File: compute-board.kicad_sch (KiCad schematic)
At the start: 5 parts, among them J1 PC104

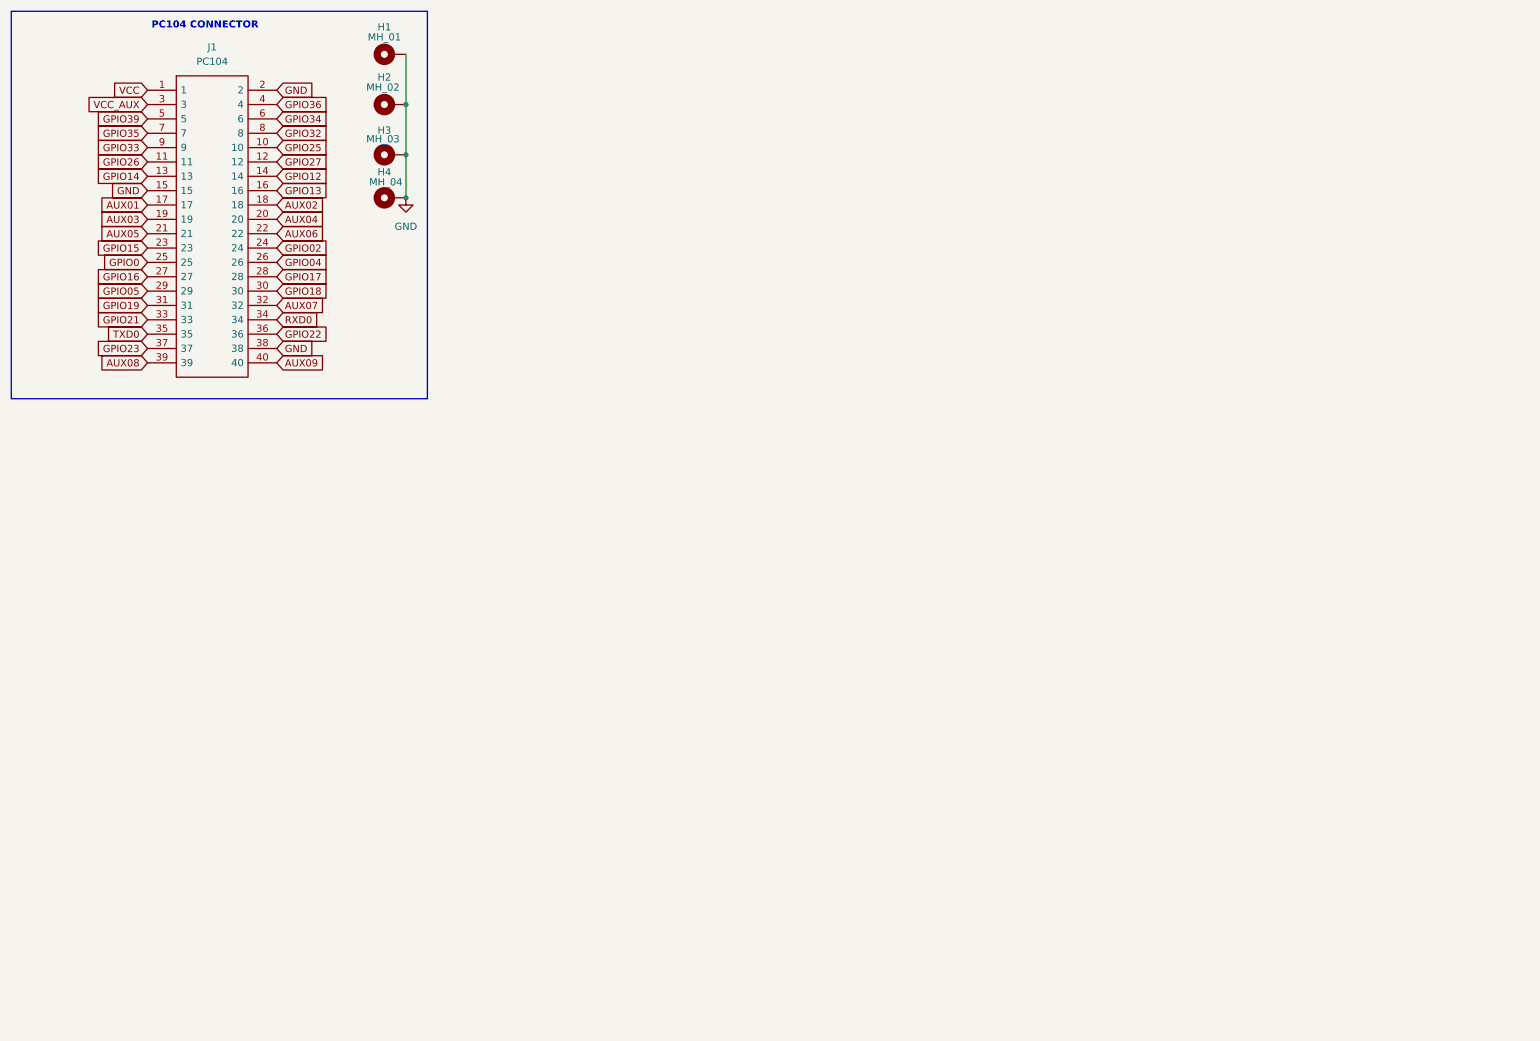
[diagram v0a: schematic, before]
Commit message: Initial commit
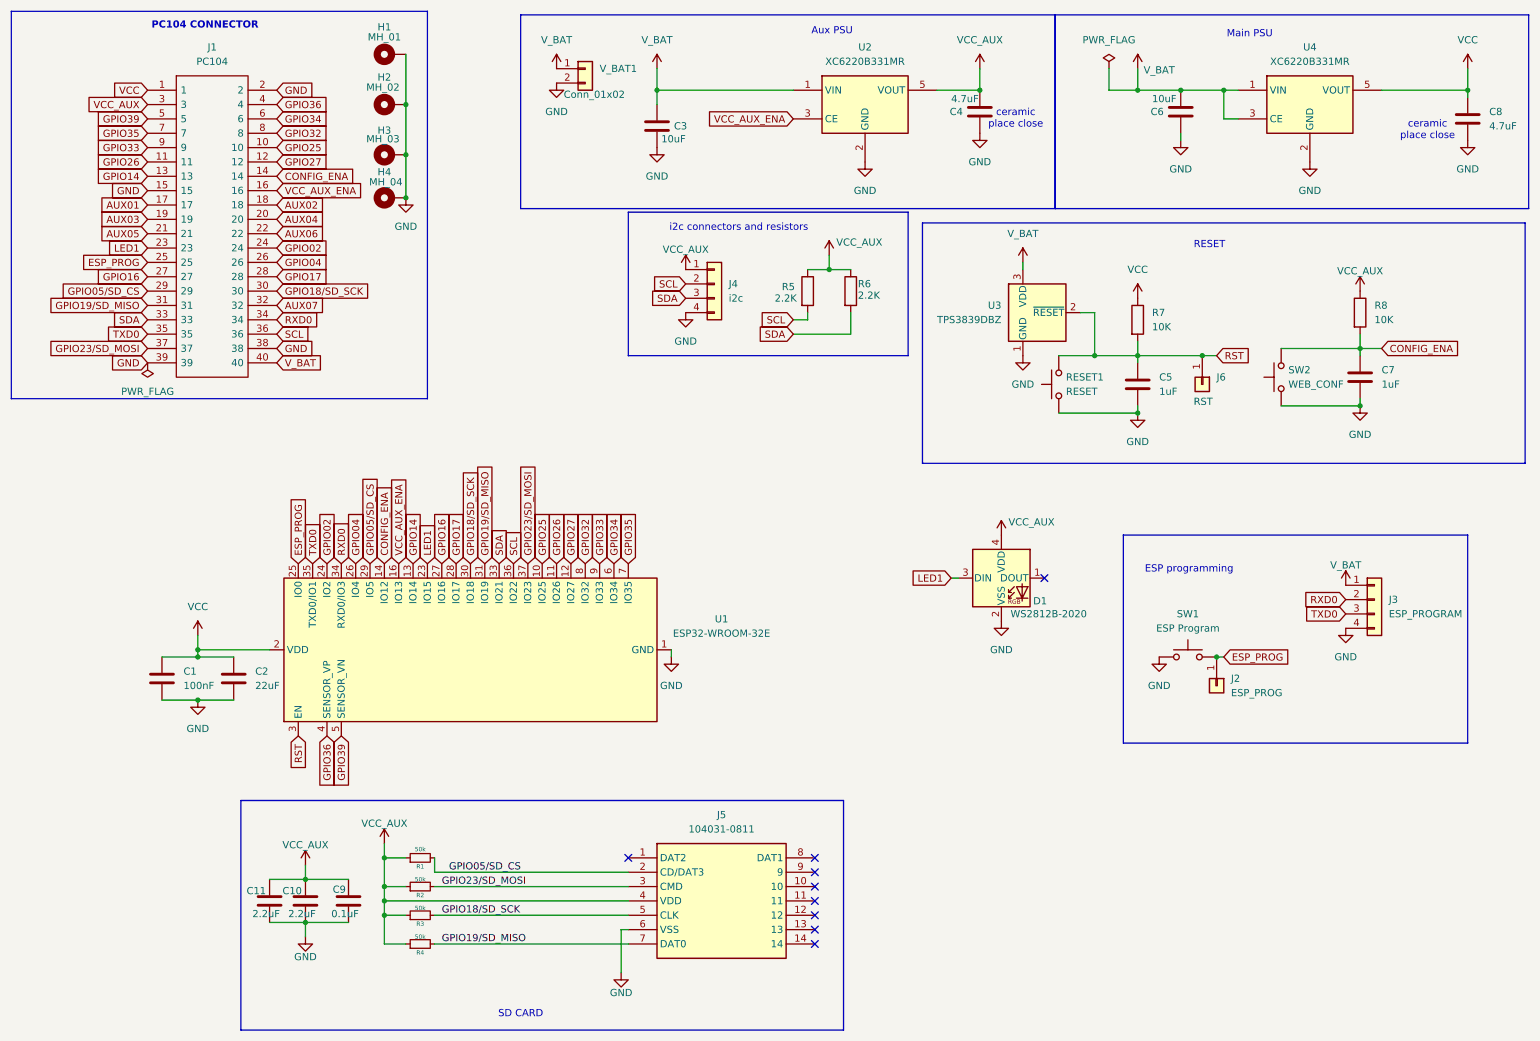
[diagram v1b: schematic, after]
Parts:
- added C1: 100nF, Capacitor_SMD:C_1206_3216Metric_Pad1.33x1.80mm_HandSolder, symbol Device:C
- added C10, C11: 2.2uF, Capacitor_SMD:C_1206_3216Metric_Pad1.33x1.80mm_HandSolder, symbol Device:C
- added C2: 22uF, Capacitor_Tantalum_SMD:CP_EIA-3528-21_Kemet-B_HandSolder, symbol Device:C
- added C3, C6: 10uF, Capacitor_SMD:C_1206_3216Metric_Pad1.33x1.80mm_HandSolder, symbol Device:C
- added C4, C8: 4.7uF, Capacitor_SMD:C_1206_3216Metric_Pad1.33x1.80mm_HandSolder, symbol Device:C
- added C5, C7: 1uF, Capacitor_SMD:C_1206_3216Metric_Pad1.33x1.80mm_HandSolder, symbol Device:C
- added C9: 0.1uF, Capacitor_SMD:C_1206_3216Metric_Pad1.33x1.80mm_HandSolder, symbol Device:C
- added D1: WS2812B-2020, LED_SMD:LED_WS2812B-2020_PLCC4_2.0x2.0mm, symbol LED:WS2812B-2020
- added J2: ESP_PROG, TestPoint:TestPoint_Pad_2.0x2.0mm, symbol Connector_Generic:Conn_01x01
- added J3: ESP_PROGRAM, Connector_JST:JST_XH_B4B-XH-AM_1x04_P2.50mm_Vertical, symbol Connector_Generic:Conn_01x04
- added J4: i2c, Connector_JST:JST_XH_B4B-XH-AM_1x04_P2.50mm_Vertical, symbol Connector_Generic:Conn_01x04
- added J5: 104031-0811, Project-Specific:1040310811, symbol MOLEX 1040310811:104031-0811
- added J6: RST, TestPoint:TestPoint_Pad_2.0x2.0mm, symbol Connector_Generic:Conn_01x01
- added R1, R2, R3, R4: 50k, Resistor_SMD:R_1206_3216Metric_Pad1.30x1.75mm_HandSolder, symbol Device:R_Small
- added R5, R6: 2.2K, Resistor_SMD:R_1206_3216Metric_Pad1.30x1.75mm_HandSolder, symbol Device:R
- added R7, R8: 10K, Resistor_SMD:R_1206_3216Metric_Pad1.30x1.75mm_HandSolder, symbol Device:R
- added RESET1: RESET, Button_Switch_SMD:SW_Push_1P1T_XKB_TS-1187A, symbol Switch:SW_Push
- added SW1: ESP Program, Button_Switch_SMD:SW_Push_1P1T_XKB_TS-1187A, symbol Switch:SW_Push
- added SW2: WEB_CONF, Button_Switch_SMD:SW_Push_1P1T_XKB_TS-1187A, symbol Switch:SW_Push
- added U1: ESP32-WROOM-32E, RF_Module:ESP32-WROOM-32D, symbol RF_Module:ESP32-WROOM-32E
- added U2, U4: XC6220B331MR, Package_TO_SOT_SMD:SOT-23-5, symbol Regulator_Linear:XC6220B331MR
- added U3: TPS3839DBZ, Package_TO_SOT_SMD:SOT-23, symbol Power_Supervisor:TPS3839DBZ
- added V_BAT1: Conn_01x02, TerminalBlock_Altech:Altech_AK300_1x02_P5.00mm_45-Degree, symbol Connector_Generic:Conn_01x02
- J1: footprint RHDR40W66P254_2X20_5146X500X1105P -> Project-Specific:RHDR40W66P254_2X20_5146X500X1105P
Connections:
- net AUX08 is gone; now on net GND: J1.39
- net GND: now also C1.2, C10.2, C11.2, C2.2, C3.1, C4.2, C5.2, C6.2, C7.2, C8.2, C9.2, D1.2 (VSS), J3.4 (Pin_4), J4.4 (Pin_4), J5.6 (VSS), RESET1.1, SW1.1, SW2.1, U1.1 (GND), U1.15 (GND), U1.38 (GND), U1.39 (GND), U2.2 (GND), U3.1 (GND), U4.2 (GND), V_BAT1.2 (Pin_2)
- net GPIO02: now also U1.24 (IO2)
- net GPIO04: now also U1.26 (IO4)
- net GPIO14: now also U1.13 (IO14)
- net GPIO16: now also U1.27 (IO16)
- net GPIO17: now also U1.28 (IO17)
- net GPIO25: now also U1.10 (IO25)
- net GPIO26: now also U1.11 (IO26)
- net GPIO27: now also U1.12 (IO27)
- net GPIO32: now also U1.8 (IO32)
- net GPIO33: now also U1.9 (IO33)
- net GPIO34: now also U1.6 (IO34)
- net GPIO35: now also U1.7 (IO35)
- net GPIO36: now also U1.4 (SENSOR_VP)
- net GPIO39: now also U1.5 (SENSOR_VN)
- net RXD0: now also J3.2 (Pin_2), U1.34 (RXD0/IO3)
- net TXD0: now also J3.3 (Pin_3), U1.35 (TXD0/IO1)
- net VCC: now also C1.1, C2.1, C8.1, R7.1, U1.2 (VDD), U4.5 (VOUT)
- net VCC_AUX: now also C10.1, C11.1, C4.1, C9.1, D1.4 (VDD), J4.1 (Pin_1), J5.4 (VDD), R1.1, R2.1, R3.1, R4.1, R5.1, R6.1, R8.1, U2.5 (VOUT)
- net AUX09 renamed V_BAT
- net V_BAT: now also C3.2, C6.1, J3.1 (Pin_1), U2.1 (VIN), U3.3 (VDD), U4.1 (VIN), U4.3 (CE), V_BAT1.1 (Pin_1)
- net GPIO0 renamed ESP_PROG
- net ESP_PROG: now also J2.1 (Pin_1), SW1.2, U1.25 (IO0)
- net GPIO05 renamed GPIO05/SD_CS
- net GPIO05/SD_CS: now also J5.2 (CD/DAT3), R1.2, U1.29 (IO5)
- net GPIO12 renamed CONFIG_ENA
- net CONFIG_ENA: now also C7.1, R8.2, SW2.2, U1.14 (IO12)
- net GPIO13 renamed VCC_AUX_ENA
- net VCC_AUX_ENA: now also U1.16 (IO13), U2.3 (CE)
- net GPIO15 renamed LED1
- net LED1: now also D1.3 (DIN), U1.23 (IO15)
- net GPIO18 renamed GPIO18/SD_SCK
- net GPIO18/SD_SCK: now also J5.5 (CLK), R3.2, U1.30 (IO18)
- net GPIO19 renamed GPIO19/SD_MISO
- net GPIO19/SD_MISO: now also J5.7 (DAT0), R4.2, U1.31 (IO19)
- net GPIO21 renamed SDA
- net SDA: now also J4.3 (Pin_3), R6.2, U1.33 (IO21)
- net GPIO22 renamed SCL
- net SCL: now also J4.2 (Pin_2), R5.2, U1.36 (IO22)
- net GPIO23 renamed GPIO23/SD_MOSI
- net GPIO23/SD_MOSI: now also J5.3 (CMD), R2.2, U1.37 (IO23)
- new net RST: C5.1, J6.1 (Pin_1), R7.2, RESET1.2, U1.3 (EN), U3.2 (~{RESET})
- no-connect marks 0 -> 9
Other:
- note added: "Aux PSU"
- note added: "ESP programming"
- note added: "Main PSU"
- note added: "RESET"
- note added: "SD CARD"
- note added: "ceramic place close"
- note added: "i2c connectors and resistors"
